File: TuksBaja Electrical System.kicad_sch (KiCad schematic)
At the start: 9 parts, among them U1 LM358, U2 A1104xLH, U3 ESP32-S3-WROOM-1, U4 A1104xLH, U5 LM358

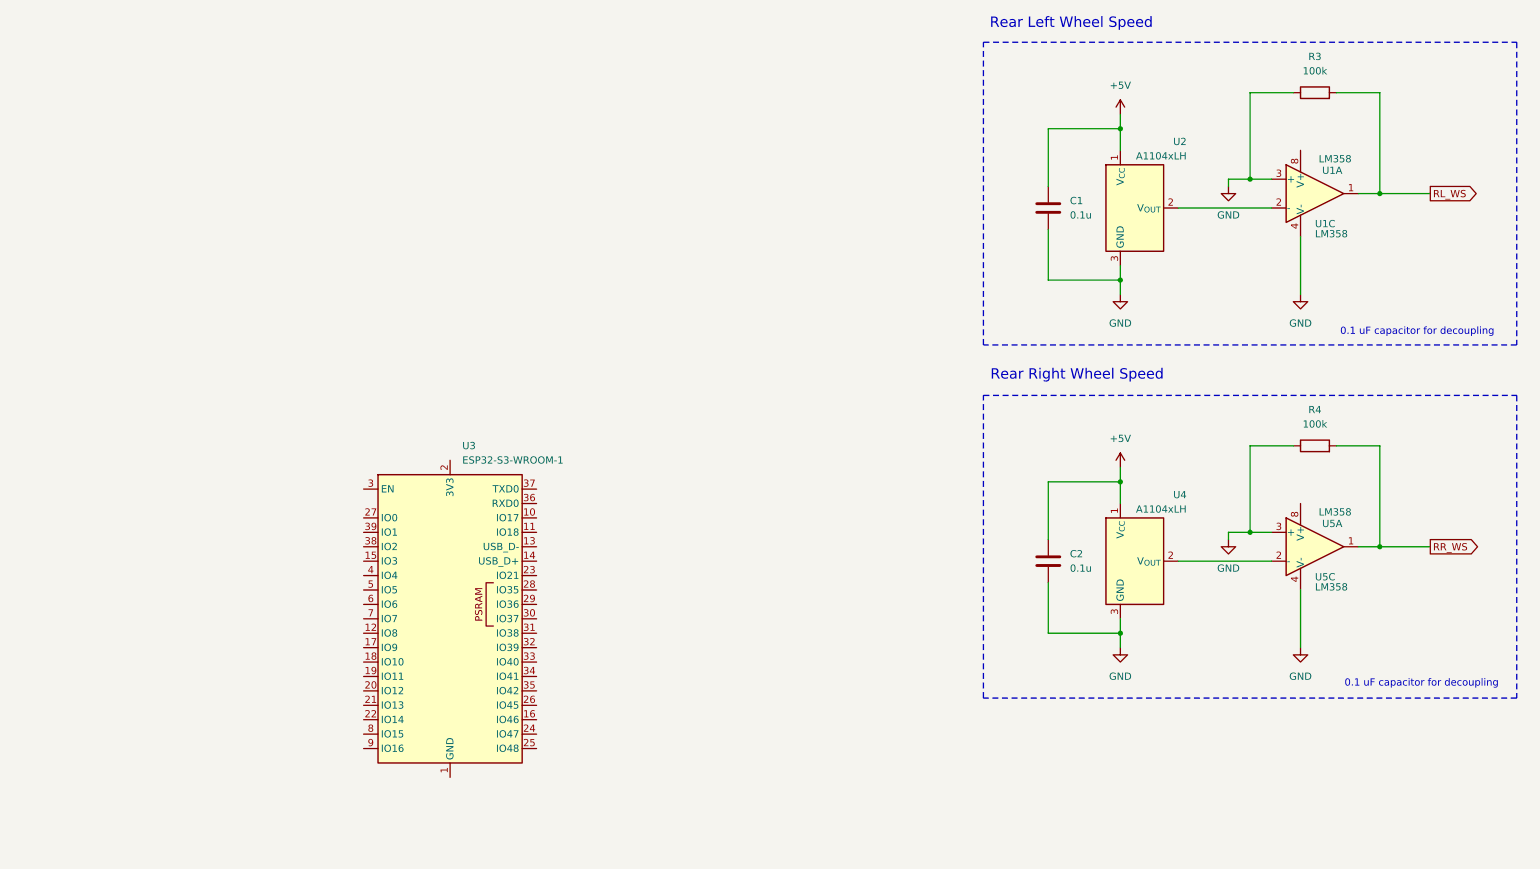
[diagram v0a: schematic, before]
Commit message: Overhall Schematic
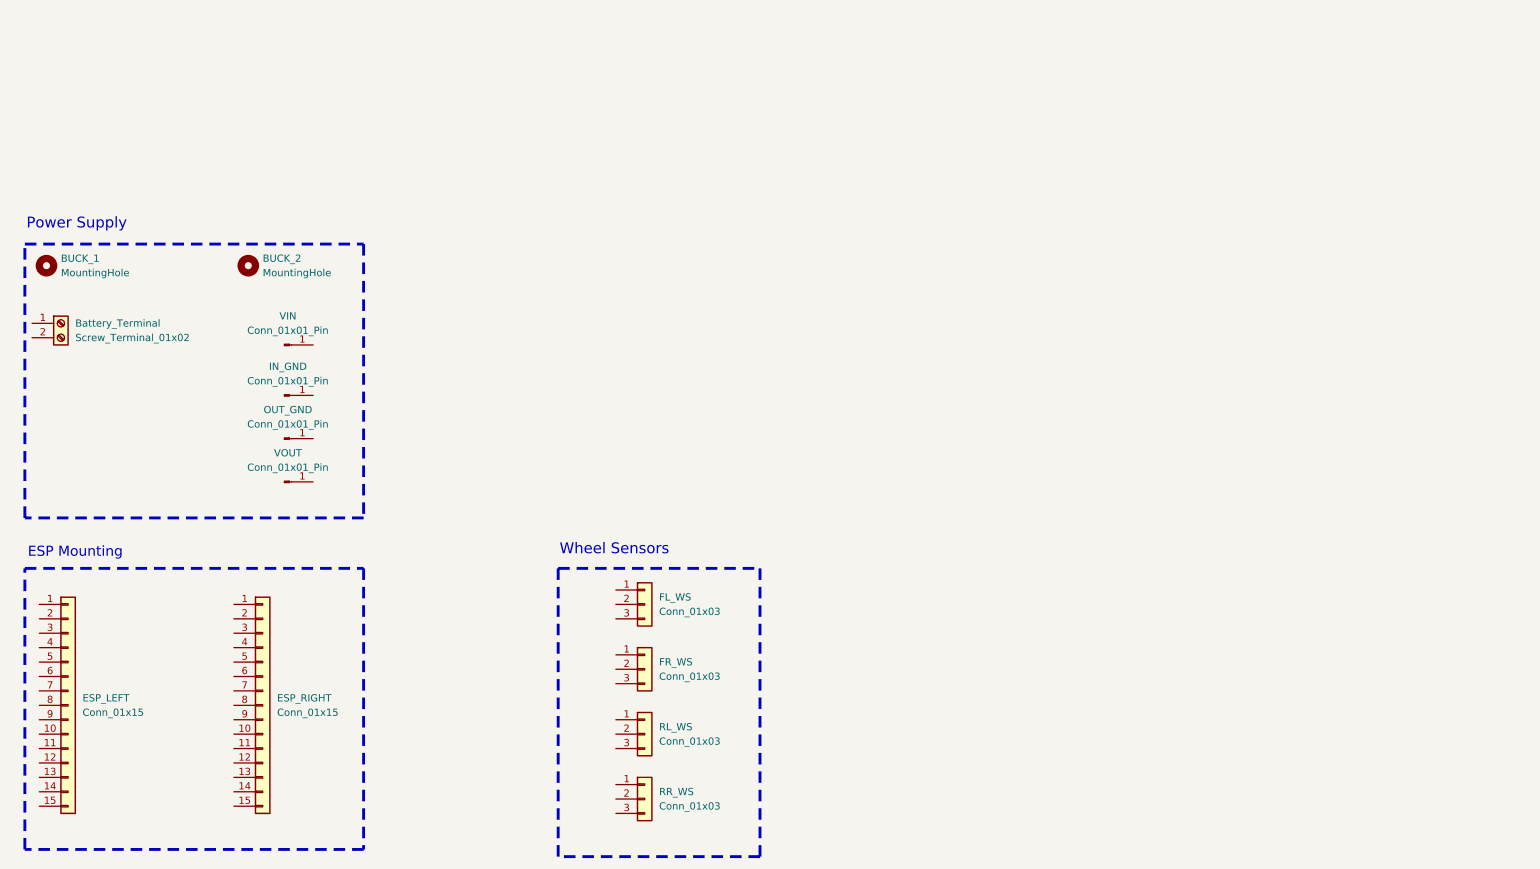
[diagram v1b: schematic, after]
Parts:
- removed C1, C2: 0.1u, symbol Device:C
- removed R3, R4: 100k, symbol Device:R
- removed U1, U5: LM358, symbol Amplifier_Operational:LM358
- removed U2, U4: A1104xLH, Package_TO_SOT_SMD:SOT-23W, symbol Sensor_Magnetic:A1104xLH
- removed U3: ESP32-S3-WROOM-1, RF_Module:ESP32-S3-WROOM-1, symbol RF_Module:ESP32-S3-WROOM-1
- added BUCK_1, BUCK_2: MountingHole, symbol Mechanical:MountingHole
- added Battery_Terminal: Screw_Terminal_01x02, symbol Connector:Screw_Terminal_01x02
- added ESP_LEFT, ESP_RIGHT: Conn_01x15, symbol Connector_Generic:Conn_01x15
- added FL_WS, FR_WS, RL_WS, RR_WS: Conn_01x03, symbol Connector_Generic:Conn_01x03
- added IN_GND, OUT_GND, VIN, VOUT: Conn_01x01_Pin, symbol Connector:Conn_01x01_Pin
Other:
- note added: "ESP Mounting"
- note added: "Power Supply"
- note added: "Wheel Sensors"
- note removed: "0.1 uF capacitor for decoupling"
- note removed: "Rear Left Wheel Speed"
- note removed: "Rear Right Wheel Speed"
